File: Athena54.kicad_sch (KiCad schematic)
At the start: 1 part

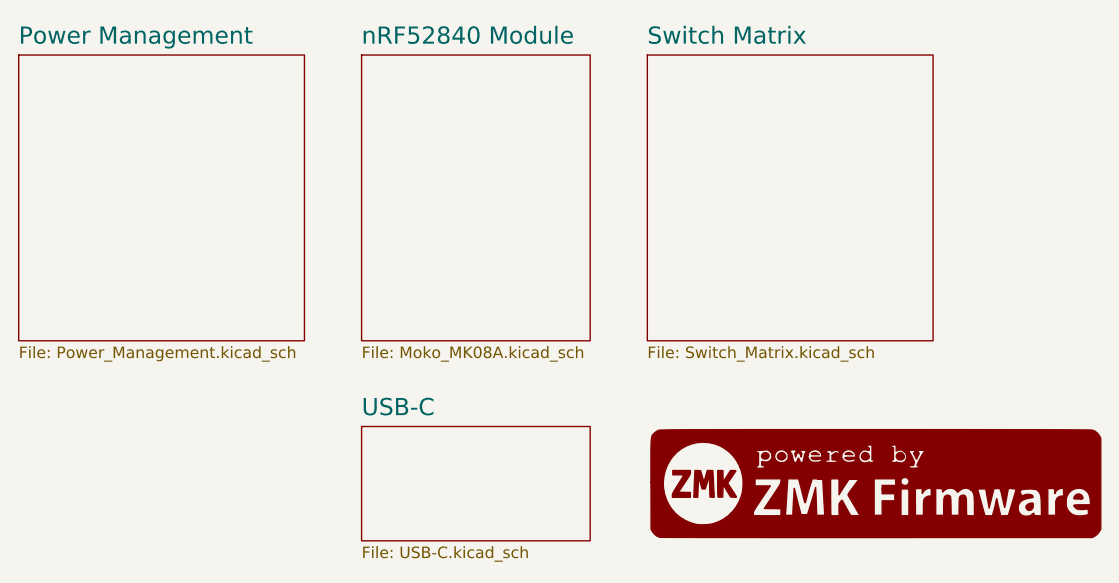
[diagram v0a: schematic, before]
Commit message: feat(pcb): Version 0.2
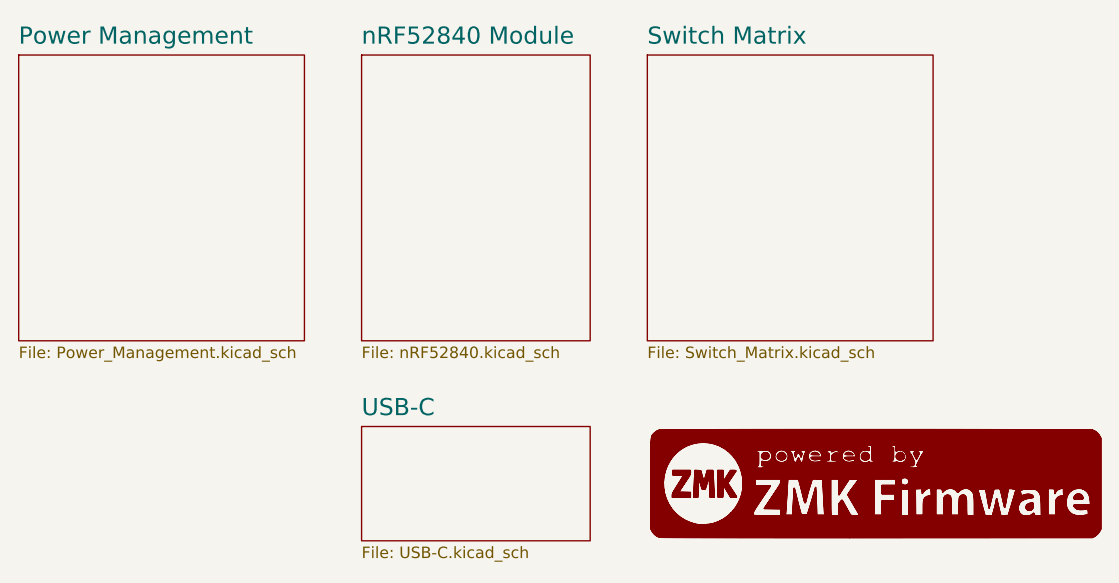
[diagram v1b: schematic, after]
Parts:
- added G2: (no value), symbol Athena54:Powered_by_ZMK_(Large)
- G1: value LOGO -> (none); footprint Athena54:Powered_By_ZMK (Large) -> (none); symbol Conejo:LOGO -> Athena54:Powered_by_ZMK_(Large)
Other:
- sheet nRF52840 Module: file Moko_MK08A.kicad_sch -> nRF52840.kicad_sch

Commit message: feat(pcb): Version 0.2.1
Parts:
- G1, G2: value (none) -> LOGO; footprint (none) -> Athena54:Powered_By_ZMK (Large)
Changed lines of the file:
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@@
       (effects (font (size 1.27 1.27)) hide)
     )
-    (property "Value" "" (id 1) (at 114.3 69.0412 0)
-      (effects (font (size 1.27 1.27)) hide)
-    )
-    (property "Footprint" "" (id 2) (at 114.3 66.675 0)
+    (property "Value" "LOGO" (id 1) (at 114.3 69.0412 0)
+      (effects (font (size 1.27 1.27)) hide)
+    )
+    (property "Footprint" "Athena54:Powered_By_ZMK (Large)" (id 2) (at 114.3 66.675 0)
       (effects (font (size 1.27 1.27)) hide)
     )
@@
       (effects (font (size 1.27 1.27)) hide)
     )
-    (property "Value" "" (id 1) (at 114.3 69.0412 0)
-      (effects (font (size 1.27 1.27)) hide)
-    )
-    (property "Footprint" "" (id 2) (at 114.3 66.675 0)
+    (property "Value" "LOGO" (id 1) (at 114.3 69.0412 0)
+      (effects (font (size 1.27 1.27)) hide)
+    )
+    (property "Footprint" "Athena54:Powered_By_ZMK (Large)" (id 2) (at 114.3 66.675 0)
       (effects (font (size 1.27 1.27)) hide)
     )
@@
     )
     (path "/0b39595e-c164-40ee-b714-5b1f9f72ce37/d7b37770-2a68-4af3-89cc-912487a95b7c"
-      (reference "F2") (unit 1) (value "500mA") (footprint "Fuse:Fuse_0402_1005Metric")
+      (reference "F2") (unit 1) (value "500mA") (footprint "Fuse:Fuse_0603_1608Metric")
     )
     (path "/0b39595e-c164-40ee-b714-5b1f9f72ce37/f7c5811e-1057-4d7b-b684-e9cae43a3f97"
@@
     )
     (path "/1803c616-4a91-454a-85d9-d17a70de9e60/263a0999-f2e0-410a-b264-fedd2638797a"
-      (reference "SW1") (unit 1) (value "POWER") (footprint "Athena54:SW_SPDT_PCM12 (Reversible)")
+      (reference "SW1") (unit 1) (value "POWER") (footprint "Athena54:SW_MSK12C02-HB (Reversible)")
     )
     (path "/122ac6b9-652b-4473-a02b-83c4af423491/bda483af-37b3-440d-b1a7-9004c33927ec"

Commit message: fix(schematic): Fix links to footprints
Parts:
- G1: value LOGO -> (none)
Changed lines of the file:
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@@
       (effects (font (size 1.27 1.27)) hide)
     )
-    (property "Value" "LOGO" (id 1) (at 114.3 69.0412 0)
+    (property "Value" "" (id 1) (at 114.3 69.0412 0)
       (effects (font (size 1.27 1.27)) hide)
     )
@@
     )
     (path "/a6c855a7-3fa9-426b-8144-57b4803ad800/79c89361-cab9-44b2-ac22-93b8e96586d9"
-      (reference "H1") (unit 1) (value "MountingHole") (footprint "Athena54:MountingHole_4.3mm")
+      (reference "H1") (unit 1) (value "4.3mm") (footprint "Athena54:MountingHole_4.3mm")
     )
     (path "/a6c855a7-3fa9-426b-8144-57b4803ad800/403df5c3-9296-4e57-9eb2-73ccbcd04e94"
-      (reference "H2") (unit 1) (value "MountingHole") (footprint "Athena54:MountingHole_4.3mm")
+      (reference "H2") (unit 1) (value "4.3mm") (footprint "Athena54:MountingHole_4.3mm")
     )
     (path "/a6c855a7-3fa9-426b-8144-57b4803ad800/8c76b6f5-ee3a-4ad1-bdeb-0ae5ad222b2c"
-      (reference "H3") (unit 1) (value "MountingHole") (footprint "Athena54:MountingHole_4.3mm")
+      (reference "H3") (unit 1) (value "4.3mm") (footprint "Athena54:MountingHole_4.3mm")
     )
     (path "/a6c855a7-3fa9-426b-8144-57b4803ad800/8ac833de-53d8-418b-a186-aa3f0694de1b"
-      (reference "H4") (unit 1) (value "MountingHole") (footprint "Athena54:MountingHole_4.3mm")
+      (reference "H4") (unit 1) (value "4.3mm") (footprint "Athena54:MountingHole_4.3mm")
     )
     (path "/a6c855a7-3fa9-426b-8144-57b4803ad800/0b485980-164a-420f-aa20-9bba2db9ae3b"
-      (reference "H5") (unit 1) (value "MountingHole") (footprint "Athena54:MountingHole_4.3mm")
+      (reference "H5") (unit 1) (value "4.3mm") (footprint "Athena54:MountingHole_4.3mm")
     )
     (path "/1803c616-4a91-454a-85d9-d17a70de9e60/b6add576-f6a8-498e-abea-3e9e2e1a2be9"
